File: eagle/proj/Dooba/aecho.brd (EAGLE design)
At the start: 43.2 x 24.6 mm, 47 parts, among them J3 SJ1-3523N, P1 I2C(SCL-SDA), P2 MP3_CTL(SCKR-SDI-DREQ-RST), P3 AMP_CTL(SHDN-CLK-UPDN), P4 PWR(GND-VIN-GND), P9 AOUT_L-GND-AOUT_R, U10 CS4334, U11 LM4811PDSO-10, U12 5.0V, U7 3.3V, U9 STA013LQFP44, X2 14.7456MHz

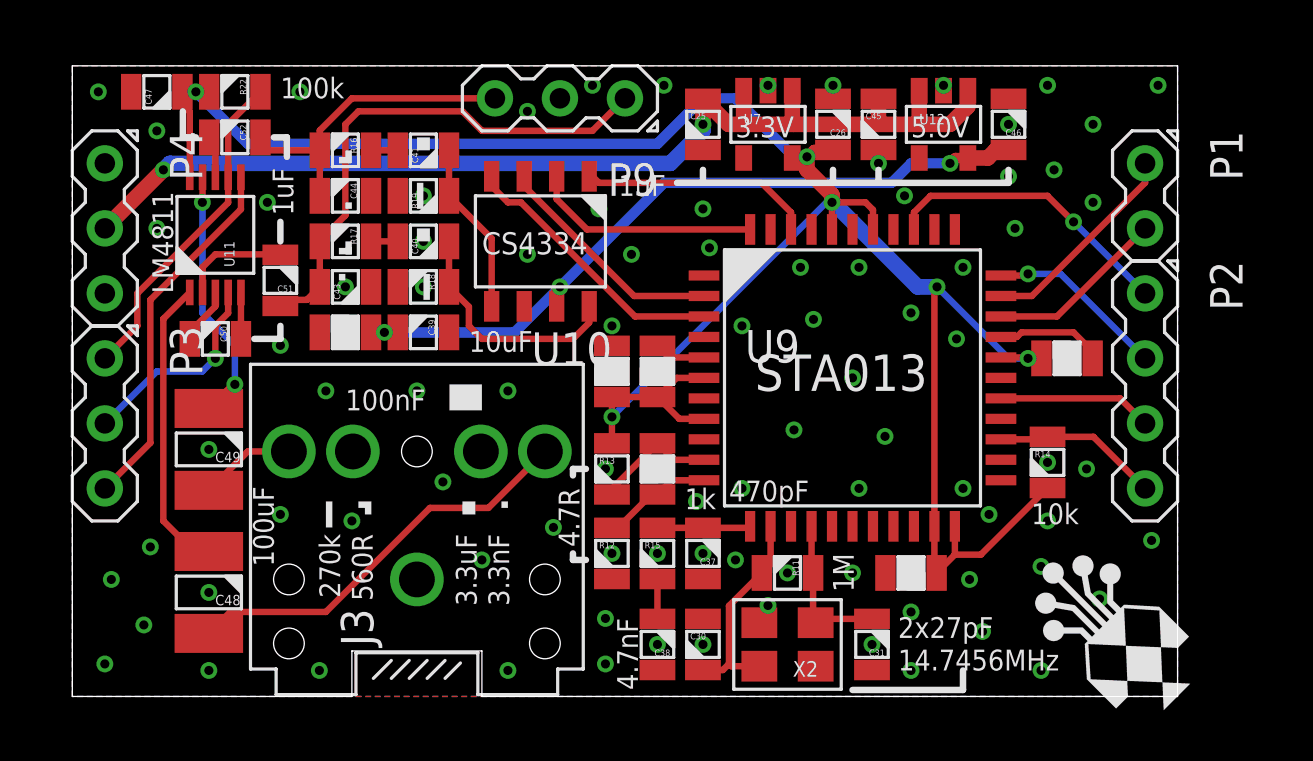
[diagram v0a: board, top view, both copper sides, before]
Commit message: Started designing Shiva mp3 player (new version)
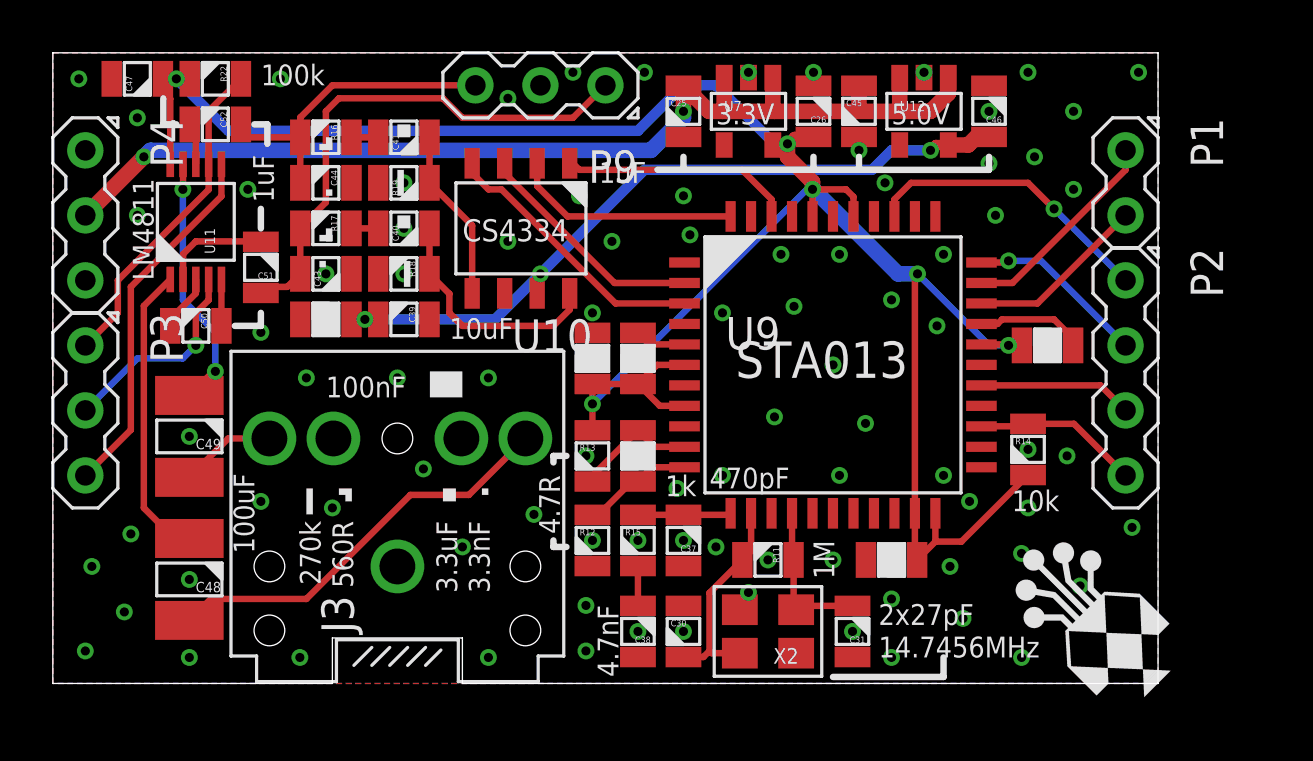
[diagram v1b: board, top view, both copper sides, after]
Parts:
- moved C25 0.92 mm to (43.7, 39.6)
- moved C26 0.92 mm to (48.8, 39.6)
- moved C32 0.92 mm to (40.1, 30.0)
- moved C33 0.92 mm to (41.9, 30.0)
- moved C40 0.92 mm to (32.8, 35.1)
- moved C43 0.92 mm to (29.7, 33.3)
- moved C45 0.92 mm to (50.5, 39.6)
- moved C46 0.92 mm to (55.6, 39.6)
- moved C52 0.92 mm to (25.4, 39.1)
- moved J3 0.92 mm to (32.5, 21.8)
- moved P3 0.92 mm to (20.3, 27.9)
- moved P4 0.92 mm to (20.3, 35.6)
- moved P9 0.92 mm to (38.1, 40.6)
- moved R17 0.92 mm to (29.7, 35.1)
- moved R18 0.92 mm to (32.8, 33.3)
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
